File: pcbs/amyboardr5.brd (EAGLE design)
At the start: 106.1 x 47.5 mm, 147 parts, among them Q2 S8050, Q5 S8050, U1 PCM9211PT, U15 H11L1SR2M, U16 SPX3819, U2 ESP32­S2­SOLO, U3 SPX3819, U4 TL074CD, U6 HX3608, Y1 22.5792MHZ

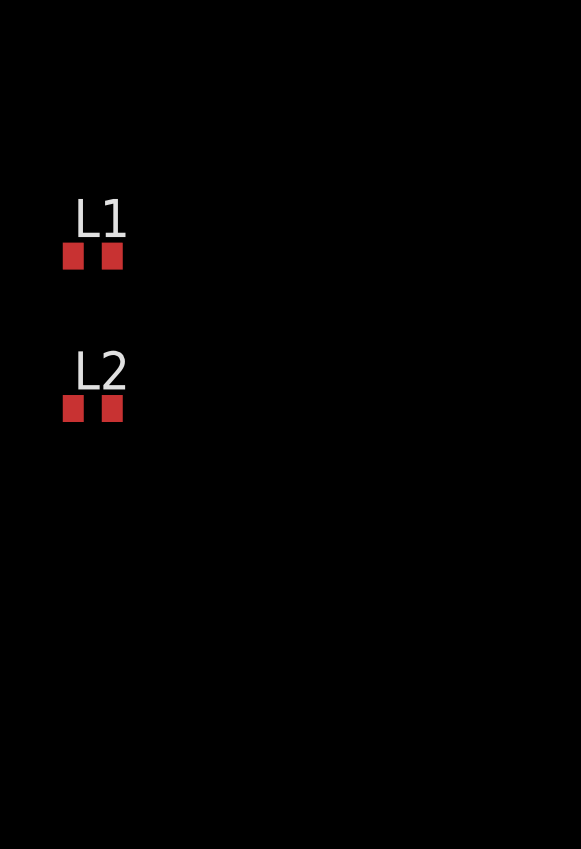
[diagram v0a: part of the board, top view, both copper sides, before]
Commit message: copying usb fb
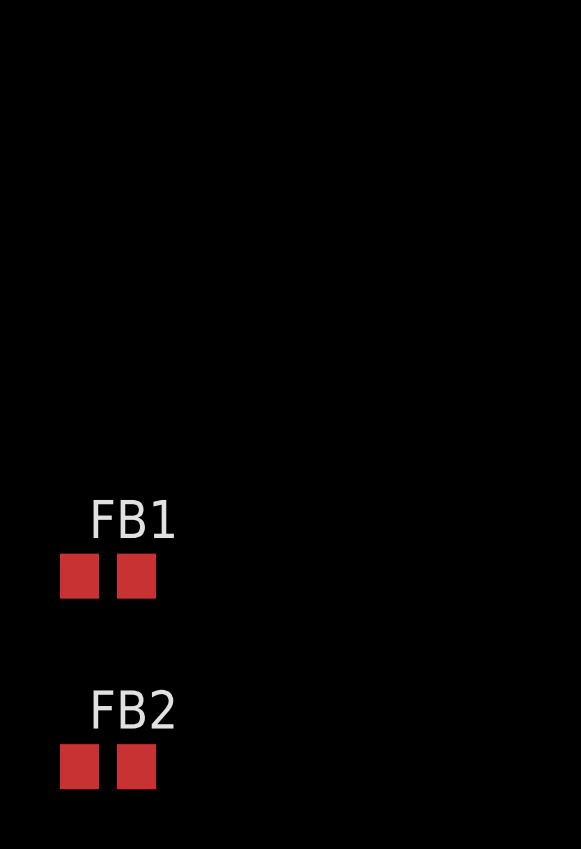
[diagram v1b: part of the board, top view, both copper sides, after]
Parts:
- removed L1, L2: BLM15HB121SN1, inductors:0402
- added FB1, FB2: 100Mhz@120R, rcl:R0805
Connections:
- net -12V: now also FB1.2; no longer L2.2
- net 12V: now also FB2.2; no longer L1.2
- net 12V_UNFILTERED: now also FB2.1; no longer L1.1
- net N$16: now also FB1.1; no longer L2.1
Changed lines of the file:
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@@
 <attribute name="VALUE" x="36.83" y="46.99" size="1.27" layer="27" rot="R90"/>
 </element>
-<element name="L1" library="inductors" library_urn="urn:adsk.eagle:library:243" package="0402" package3d_urn="urn:adsk.eagle:package:15132/1" value="BLM15HB121SN1" x="-284.226" y="-1072.388" smashed="yes">
-<attribute name="NAME" x="-284.861" y="-1071.753" size="1.27" layer="25"/>
-<attribute name="POPULARITY" value="0" x="-284.226" y="-1072.388" size="1.778" layer="27" display="off"/>
-<attribute name="VALUE" x="-284.861" y="-1074.293" size="1.27" layer="27"/>
+<element name="FB1" library="rcl" package="R0805" value="100Mhz@120R" x="-283.718" y="-1083.056" smashed="yes">
+<attribute name="NAME" x="-284.353" y="-1081.786" size="1.27" layer="25"/>
+<attribute name="VALUE" x="-284.353" y="-1085.596" size="1.27" layer="27"/>
 </element>
-<element name="L2" library="inductors" library_urn="urn:adsk.eagle:library:243" package="0402" package3d_urn="urn:adsk.eagle:package:15132/1" value="BLM15HB121SN1" x="-284.226" y="-1077.468" smashed="yes">
-<attribute name="NAME" x="-284.861" y="-1076.833" size="1.27" layer="25"/>
-<attribute name="POPULARITY" value="0" x="-284.226" y="-1077.468" size="1.778" layer="27" display="off"/>
-<attribute name="VALUE" x="-284.861" y="-1079.373" size="1.27" layer="27"/>
+<element name="FB2" library="rcl" package="R0805" value="100Mhz@120R" x="-283.718" y="-1089.406" smashed="yes">
+<attribute name="NAME" x="-284.353" y="-1088.136" size="1.27" layer="25"/>
+<attribute name="VALUE" x="-284.353" y="-1091.946" size="1.27" layer="27"/>
 </element>
 </elements>
@@
 <contactref element="C20" pad="2"/>
 <contactref element="U4" pad="11"/>
-<contactref element="L2" pad="2"/>
-<wire x1="57.593" y1="15.24" x2="-283.576" y2="-1077.468" width="0" layer="19" extent="1-1"/>
+<contactref element="FB1" pad="2"/>
+<wire x1="57.593" y1="15.24" x2="-282.768" y2="-1083.056" width="0" layer="19" extent="1-1"/>
 <wire x1="6.858" y1="33.528" x2="57.593" y2="15.24" width="0" layer="19" extent="1-1"/>
 </signal>
@@
 <contactref element="R17" pad="2"/>
 <contactref element="C28" pad="1"/>
-<contactref element="L1" pad="2"/>
-<wire x1="35.56" y1="34.036" x2="-283.576" y2="-1072.388" width="0" layer="19" extent="1-1"/>
+<contactref element="FB2" pad="2"/>
+<wire x1="35.56" y1="34.036" x2="-282.768" y2="-1089.406" width="0" layer="19" extent="1-1"/>
 <wire x1="29.972" y1="38.1" x2="35.56" y2="34.036" width="0" layer="19" extent="1-1"/>
 </signal>
@@
 <contactref element="D10" pad="A"/>
 <contactref element="C31" pad="2"/>
-<contactref element="L2" pad="1"/>
-<wire x1="17.519" y1="34.29" x2="-284.876" y2="-1077.468" width="0" layer="19" extent="1-1"/>
+<contactref element="FB1" pad="1"/>
+<wire x1="17.519" y1="34.29" x2="-284.668" y2="-1083.056" width="0" layer="19" extent="1-1"/>
 <wire x1="10.16" y1="33.528" x2="17.519" y2="34.29" width="0" layer="19" extent="1-1"/>
 </signal>
 <signal name="12V_UNFILTERED">
 <contactref element="C27" pad="1"/>
-<contactref element="L1" pad="1"/>
 <contactref element="D8" pad="C"/>
 <contactref element="U3" pad="1"/>
@@
 <contactref element="U$7" pad="5"/>
 <contactref element="C26" pad="1"/>
-<wire x1="51.054" y1="24.07" x2="-284.876" y2="-1072.388" width="0" layer="19" extent="1-1"/>
+<contactref element="FB2" pad="1"/>
+<wire x1="51.054" y1="24.07" x2="-284.668" y2="-1089.406" width="0" layer="19" extent="1-1"/>
 <wire x1="38.034" y1="21.0519" x2="51.054" y2="24.07" width="0" layer="19" extent="1-1"/>
 <wire x1="38.107" y1="20.574" x2="38.034" y2="21.0519" width="0" layer="19" extent="1-1"/>
